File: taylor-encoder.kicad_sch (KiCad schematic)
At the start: 35 parts, among them T4 T50_COMBINER, U3 FST3253, U4 LM4562, U5 LM4562

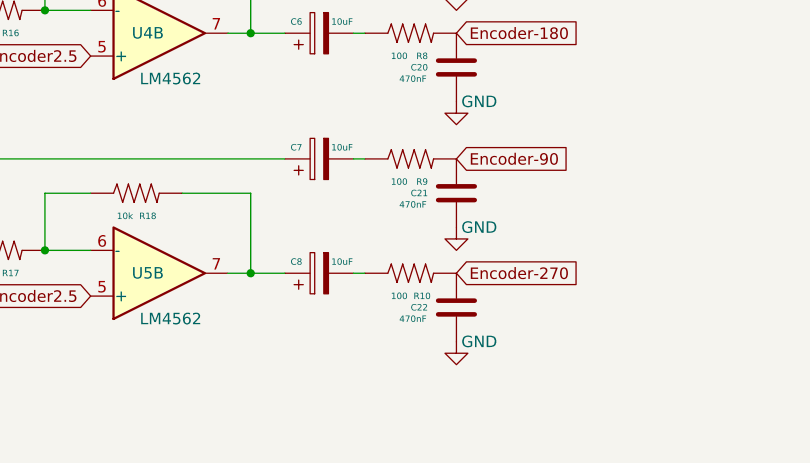
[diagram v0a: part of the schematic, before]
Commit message: gg
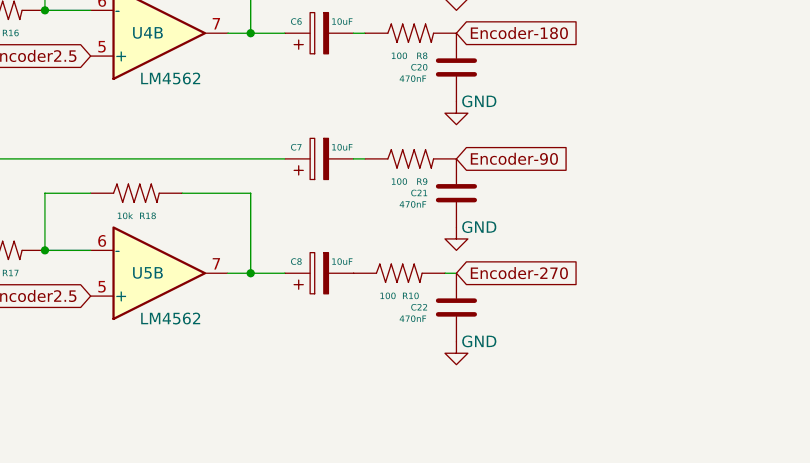
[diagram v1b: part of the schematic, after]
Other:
- moved on the sheet: R10
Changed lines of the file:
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@@
   (junction (at 85.09 60.96) (diameter 0) (color 0 0 0 0)
   )
-  (wire (pts (xy 119.38 132.08) (xy 120.65 132.08))
-    (stroke (width 0) (type default) (color 0 0 0 0))
-  )
   (wire (pts (xy 107.95 105.41) (xy 107.95 96.52))
     (stroke (width 0) (type default) (color 0 0 0 0))
@@
   )
   (wire (pts (xy 201.93 130.81) (xy 203.2 130.81))
+    (stroke (width 0) (type default) (color 0 0 0 0))
+  )
+  (wire (pts (xy 129.54 132.08) (xy 130.81 132.08))
     (stroke (width 0) (type default) (color 0 0 0 0))
   )
@@
     (pin "1")
   )
-  (symbol (lib_id "Xenir:Resistor") (at 125.73 132.08 0) (unit 1)
-    (in_bom yes) (on_board yes)
-    (property "Reference" "R10" (id 0) (at 127 134.62 0)
-      (effects (font (size 0.7112 0.7112)))
-    )
-    (property "Value" "100" (id 1) (at 124.46 134.62 0)
-      (effects (font (size 0.7112 0.7112)))
-    )
-    (property "Footprint" "Resistor_SMD:R_0805_2012Metric" (id 2) (at 125.73 134.62 0)
-      (effects (font (size 1.27 1.27)) hide)
-    )
-    (property "Datasheet" "" (id 3) (at 125.73 134.62 0)
-      (effects (font (size 1.27 1.27)) hide)
-    )
+  (symbol (lib_id "Xenir:Resistor") (at 124.46 132.08 0) (unit 1)
+    (in_bom yes) (on_board yes)
+    (property "Reference" "R10" (id 0) (at 125.73 134.62 0)
+      (effects (font (size 0.7112 0.7112)))
+    )
+    (property "Value" "100" (id 1) (at 123.19 134.62 0)
+      (effects (font (size 0.7112 0.7112)))
+    )
+    (property "Footprint" "Resistor_SMD:R_0805_2012Metric" (id 2) (at 124.46 134.62 0)
+      (effects (font (size 1.27 1.27)) hide)
+    )
+    (property "Datasheet" "" (id 3) (at 124.46 134.62 0)
+      (effects (font (size 1.27 1.27)) hide)
+    )
